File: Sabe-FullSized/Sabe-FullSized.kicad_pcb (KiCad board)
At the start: 4 copper layers, 67.9 x 86.3 mm, 33 parts, among them J1 Roboteq, J10 Misc 4, J11 Conn_01x02, J2 Serial 1, J3 Serial 2, J4 Serial 3, J5 5V, J6 Conn_01x02, J7 Misc 1, J8 Misc 2, J9 Misc 3, U1 LM2937xT, U5 ESP32-S3-DEVKITC-1-N8R2, U7 XIAO_ESP32C3

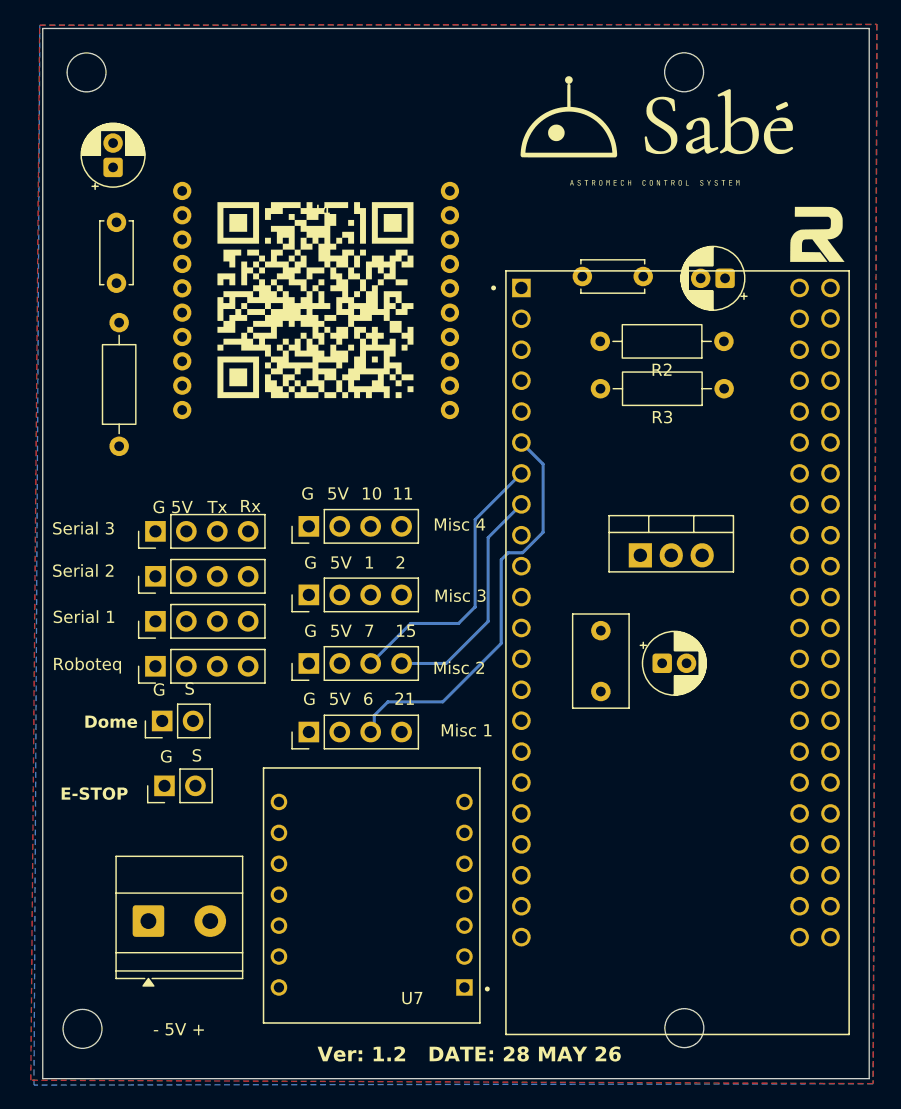
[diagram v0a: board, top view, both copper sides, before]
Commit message: sabe
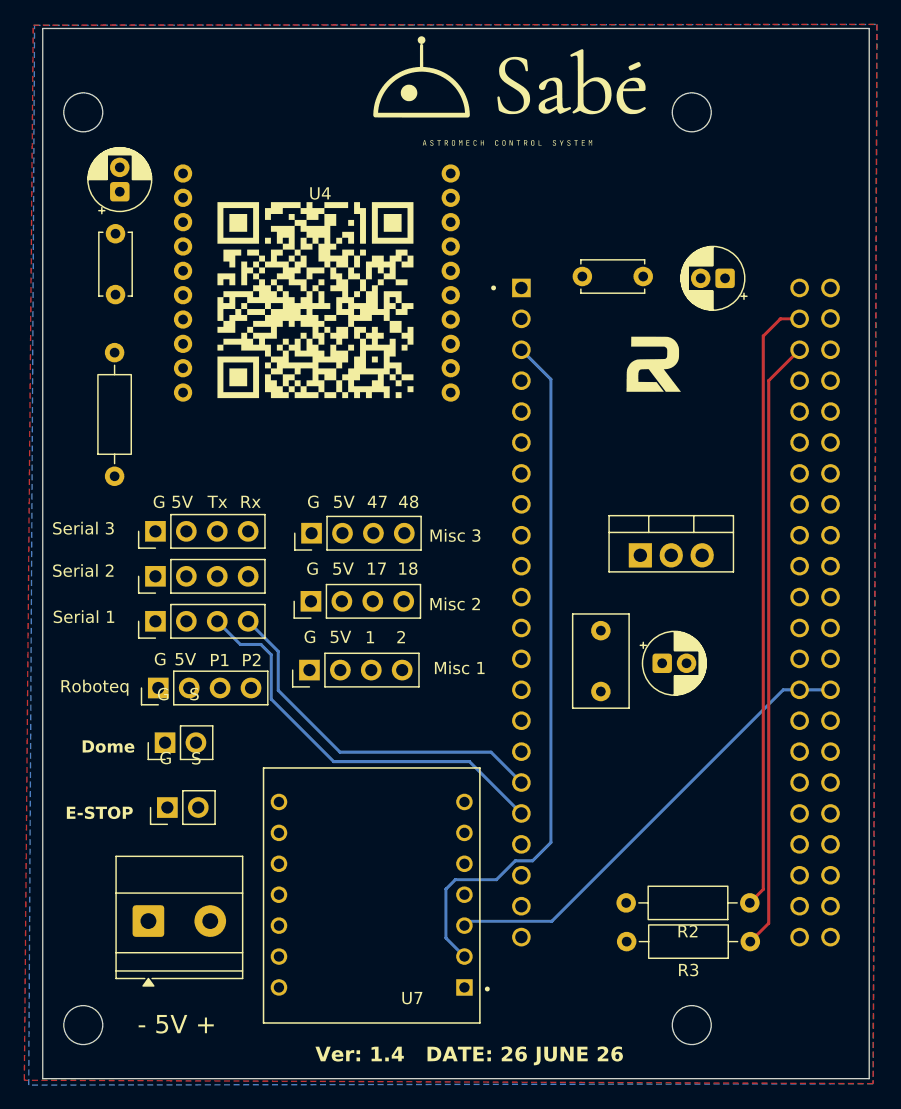
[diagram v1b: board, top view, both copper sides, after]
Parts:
- removed J10: Misc 4, Connector_PinHeader_2.54mm:PinHeader_1x04_P2.54mm_Vertical
- J6: value Conn_01x02 -> Dome PWM
- moved R2 46.2 mm to (175.8, 116.0)
- moved R3 45.5 mm to (175.8, 119.1)
- moved G*** 17.2 mm to (167.9, 72.1)
- moved G*** 12.5 mm to (155.9, 49.2)
- moved J8 5.11 mm to (139.7, 91.2)
- moved J7 5.09 mm to (139.6, 96.8)
- moved J9 5.07 mm to (139.8, 85.6)
- moved H1 3.35 mm to (171.0, 51.0)
- moved H2 3.29 mm to (121.0, 51.0)
- moved R1 2.49 mm to (123.6, 80.9)
- moved C4 2.07 mm to (124.0, 57.5)
- moved J1 1.80 mm to (127.2, 98.3)
- moved J11 1.80 mm to (127.9, 108.1)
- moved J6 1.80 mm to (127.7, 102.8)
- moved U4 1.44 mm to (140.2, 64.7)
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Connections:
- J11 pad 1: unconnected-(J11-Pin_1-Pad1) -> GND
- J11 pad 2: unconnected-(J11-Pin_2-Pad2) -> ESTOP
- J4 pad 3: S3_TX -> S3_RX
- J4 pad 4: S3_RX -> S3_TX
- J6 pad 1: unconnected-(J6-Pin_1-Pad1) -> GND
- J6 pad 2: unconnected-(J6-Pin_2-Pad2) -> Dome_PWM
- J7 pad 3: Misc1_G6 -> Misc1_G1
- J7 pad 4: Misc1_G21 -> Misc1_G2
- J8 pad 3: Misc1_G7 -> Misc2_G17
- J8 pad 4: Misc1_G15 -> Misc2_G18
- J9 pad 3: Misc1_G1 -> Misc3_G47
- J9 pad 4: Misc1_G2 -> Misc3_G48
- U5 pad J1_10: xbee_din -> unconnected-(U5-GPIO17-PadJ1_10)
- U5 pad J1_11: xbee_dout -> unconnected-(U5-GPIO18-PadJ1_11)
- U5 pad J1_12: S2_RX -> RBTQ_2
- U5 pad J1_15: xbee_rst -> Dome_PWM
- U5 pad J1_16: Misc1_G10 -> ESTOP
- U5 pad J1_17: Misc1_G11 -> S1_RX
- U5 pad J1_18: unconnected-(U5-GPIO12-PadJ1_18) -> S1_TX
- U5 pad J1_19: S3_TX -> S2_RX
- U5 pad J1_20: S3_RX -> S2_TX
- U5 pad J1_4: RBTQ_1 -> xbee_dout
- U5 pad J1_5: RBTQ_2 -> xbee_din
- U5 pad J1_6: Misc1_G6 -> xbee_rst
- U5 pad J1_7: Misc1_G7 -> RBTQ_1
- U5 pad J1_8: Misc1_G15 -> S3_RX
- U5 pad J1_9: S2_TX -> S3_TX
- U5 pad J3_16: S1_RX -> Misc3_G48
- U5 pad J3_17: S1_TX -> Misc3_G47
- U5 pad J3_18: Misc1_G21 -> unconnected-(U5-GPIO21-PadJ3_18)
- U7 pad 13: unconnected-(U7-GND-Pad13) -> GND
- U7 pad 14: unconnected-(U7-VUSB-Pad14) -> 5V
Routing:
- net RST: track 0.00 -> 57.9 mm
- net S6TX_C6RX: track 0.00 -> 53.2 mm
- net S6RX_C6TX: track 0.00 -> 52.8 mm
- net Misc3_G47: track 0.00 -> 48.9 mm
- net Net-(U7-D8): track 0.00 -> 44.9 mm
- net Misc3_G48: track 0.00 -> 43.6 mm
- net Net-(U7-D9): track 0.00 -> 40.8 mm
- net GPIO_0: track 0.00 -> 38.1 mm
- net Misc1_G21: track 38.0 -> 0.00 mm
- net Misc1_G6: track 33.7 -> 0.00 mm
- net RBTQ_2: track 55.4 -> 24.4 mm
- net Misc1_G10: track 29.5 -> 0.00 mm
- net ESTOP: track 0.00 -> 28.8 mm
- net Dome_PWM: track 0.00 -> 27.5 mm
- net Misc1_G11: track 26.3 -> 0.00 mm
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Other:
- board text added: "17"
- board text added: "18"
- board text added: "47"
- board text added: "48"
- board text added: "P1"
- board text added: "P2"
- board text added: "Ver: 1.4 DATE: 26 JUNE 26"
- board text removed: "10"
- board text removed: "11"
- board text removed: "15"
- board text removed: "21"
- board text removed: "6"
- board text removed: "7"
- board text removed: "Misc 4"
- board text removed: "Ver: 1.2 DATE: 28 MAY 26"
